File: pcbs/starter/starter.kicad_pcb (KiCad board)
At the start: 2 copper layers, 62.5 x 68.5 mm, 17 parts, among them J1 Conn_01x06_Socket, J2 Relay Anschluss, J3 12V Eingang und GND, J4 Conn_01x02_Socket, Q2 2N7000, Q3 2N7000, Q4 2N7000, U1 ESP32-C3_SUPERMINI_TH

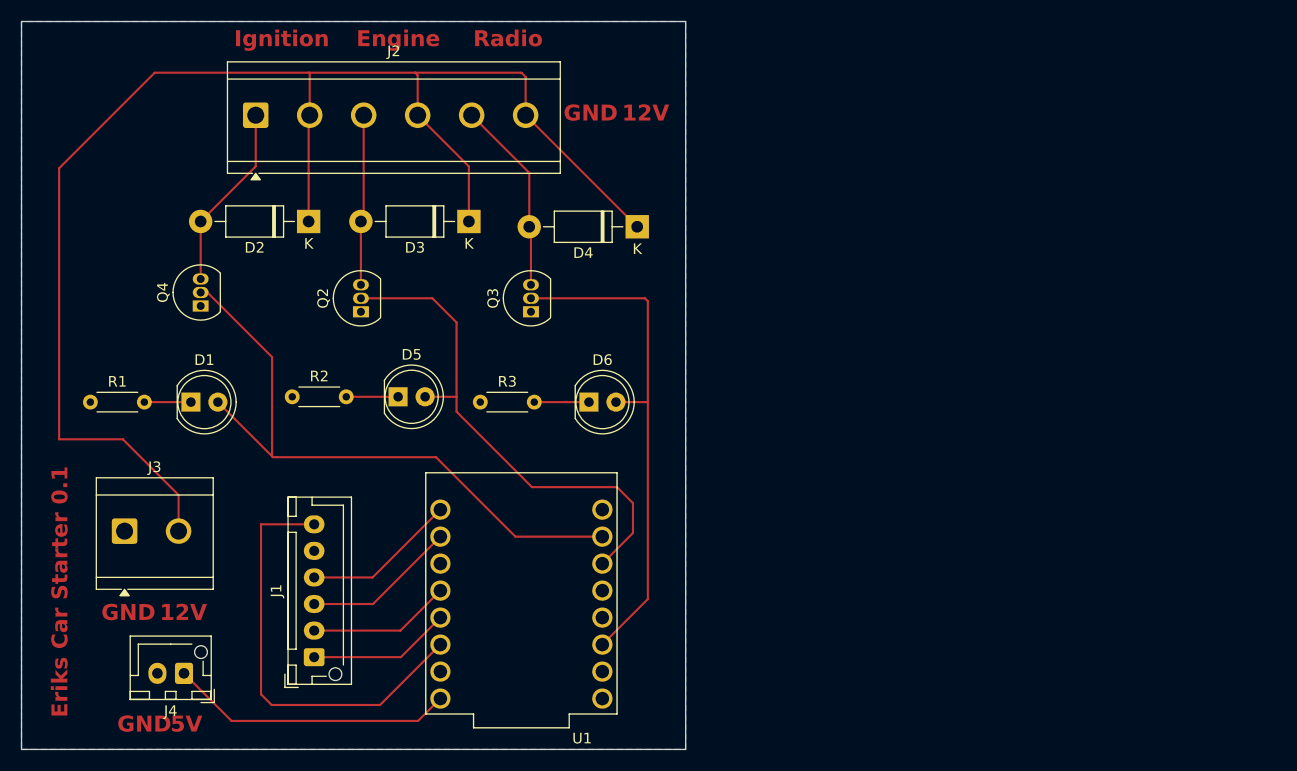
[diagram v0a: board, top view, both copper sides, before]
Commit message: first pcb revision ordered at JLCPCB
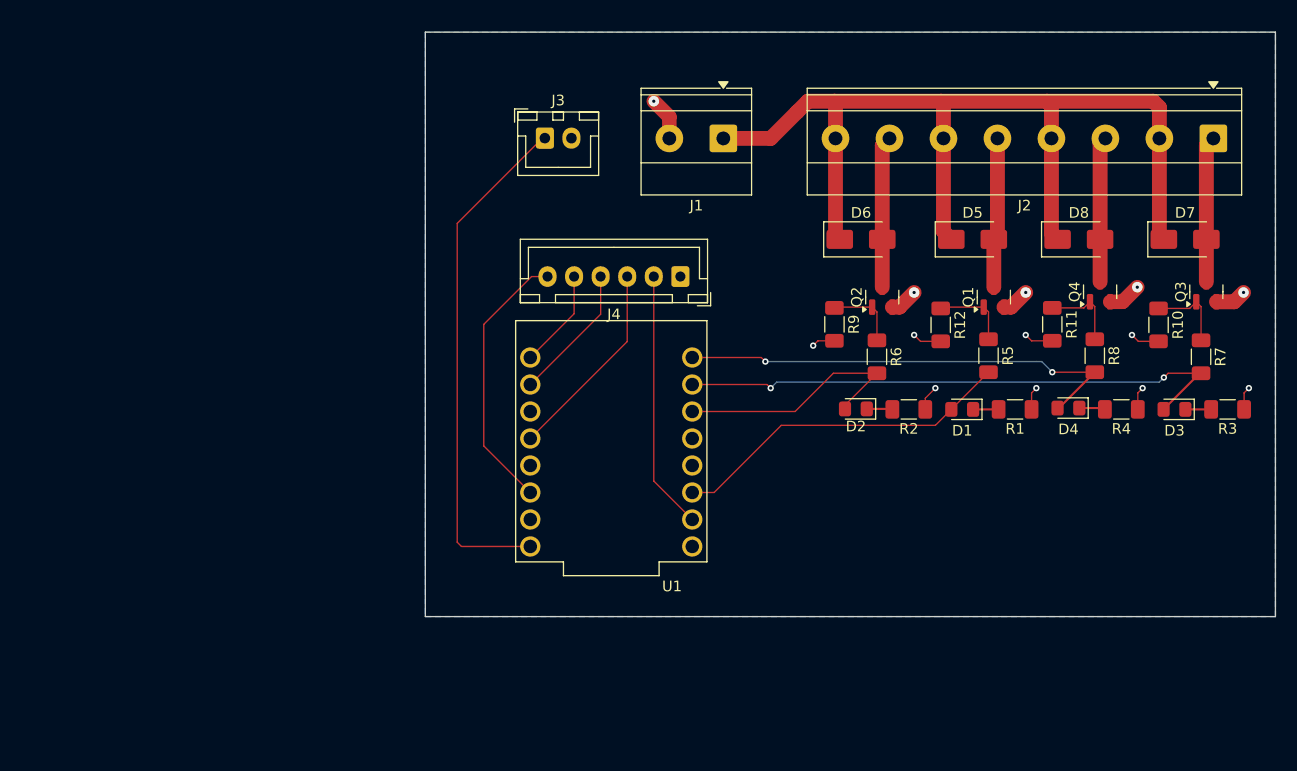
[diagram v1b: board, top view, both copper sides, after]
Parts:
- added D7: SS14, Diode_SMD:D_SMA, F.Cu at (189.0, 69.0)
- added D8: SS14, Diode_SMD:D_SMA, F.Cu at (179.0, 69.0)
- added Q1: AO3400A, Package_TO_SOT_SMD:SOT-23, F.Cu at (171.0, 74.4)
- added R10: 10k, Resistor_SMD:R_1206_3216Metric_Pad1.30x1.75mm_HandSolder, F.Cu at (186.5, 77.0)
- added R11: 10k, Resistor_SMD:R_1206_3216Metric_Pad1.30x1.75mm_HandSolder, F.Cu at (176.5, 77.0)
- added R12: 10k, Resistor_SMD:R_1206_3216Metric_Pad1.30x1.75mm_HandSolder, F.Cu at (166.0, 77.0)
- added R4: 200, Resistor_SMD:R_1206_3216Metric_Pad1.30x1.75mm_HandSolder, F.Cu at (183.0, 85.0)
- added R5: 47, Resistor_SMD:R_1206_3216Metric_Pad1.30x1.75mm_HandSolder, F.Cu at (170.5, 80.0)
- added R6: 47, Resistor_SMD:R_1206_3216Metric_Pad1.30x1.75mm_HandSolder, F.Cu at (160.0, 80.0)
- added R7: 47, Resistor_SMD:R_1206_3216Metric_Pad1.30x1.75mm_HandSolder, F.Cu at (190.5, 80.0)
- added R8: 47, Resistor_SMD:R_1206_3216Metric_Pad1.30x1.75mm_HandSolder, F.Cu at (180.5, 80.0)
- added R9: 10k, Resistor_SMD:R_1206_3216Metric_Pad1.30x1.75mm_HandSolder, F.Cu at (156.0, 77.0)
- D1: footprint LED_THT:LED_D5.0mm -> LED_SMD:LED_0805_2012Metric_Pad1.15x1.40mm_HandSolder
- D2, D3, D4: value 1N4003 -> LED; footprint Diode_THT:D_DO-41_SOD81_P10.16mm_Horizontal -> LED_SMD:LED_0805_2012Metric_Pad1.15x1.40mm_HandSolder
- D5, D6: value LED -> SS14; footprint LED_THT:LED_D5.0mm -> Diode_SMD:D_SMA
- J1: value Conn_01x06_Socket -> Power 12V; footprint Connector_JST:JST_XH_B6B-XH-AM_1x06_P2.50mm_Vertical -> TerminalBlock_Phoenix:TerminalBlock_Phoenix_MKDS-1,5-2-5.08_1x02_P5.08mm_Horizontal
- J2: value Relay Anschluss -> Relays; footprint TerminalBlock_CUI:TerminalBlock_CUI_TB007-508-06_1x06_P5.08mm_Horizontal -> TerminalBlock_Phoenix:TerminalBlock_Phoenix_MKDS-1,5-8-5.08_1x08_P5.08mm_Horizontal
- J3: value 12V Eingang und GND -> Power 5V; footprint TerminalBlock_CUI:TerminalBlock_CUI_TB007-508-02_1x02_P5.08mm_Horizontal -> Connector_JST:JST_XH_B2B-XH-A_1x02_P2.50mm_Vertical
- J4: value Conn_01x02_Socket -> Sensor Key Position; footprint Connector_JST:JST_XH_B2B-XH-AM_1x02_P2.50mm_Vertical -> Connector_JST:JST_XH_B6B-XH-A_1x06_P2.50mm_Vertical
- Q2, Q3, Q4: value 2N7000 -> AO3400A; footprint Package_TO_SOT_THT:TO-92_Inline -> Package_TO_SOT_SMD:SOT-23
- R1, R2, R3: value 200R -> 200; footprint Resistor_THT:R_Axial_DIN0204_L3.6mm_D1.6mm_P5.08mm_Horizontal -> Resistor_SMD:R_1206_3216Metric_Pad1.30x1.75mm_HandSolder
- moved J2 90.1 mm to (191.7, 59.5), turned to 180 degrees
- moved R1 87.0 mm to (173.0, 85.0), turned to 180 degrees
- moved Q4 84.7 mm to (181.0, 73.9)
- moved D1 72.6 mm to (168.0, 85.0), turned to 180 degrees
- moved R3 70.3 mm to (193.0, 85.0), turned to 180 degrees
- moved D3 68.7 mm to (188.0, 85.0)
- moved Q3 63.6 mm to (191.0, 73.9)
- moved J1 62.2 mm to (145.5, 59.5), turned to 180 degrees
- moved J4 59.8 mm to (141.5, 72.5)
- moved R2 58.0 mm to (163.0, 85.0), turned to 180 degrees
- moved D5 56.1 mm to (169.0, 69.0)
- moved D2 54.4 mm to (158.0, 85.0)
- moved J3 54.1 mm to (128.8, 59.5)
- moved Q2 49.1 mm to (160.5, 74.4)
- moved D4 44.0 mm to (178.0, 84.9)
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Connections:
- D2 pad 1: +12V -> Net-(D2-K)
- D3 pad 1: +12V -> Net-(D3-K)
- D4 pad 1: +12V -> Net-(D4-K)
- D5 pad 1: Net-(D5-K) -> +12V
- D6 pad 1: Net-(D6-K) -> +12V
- J1 pad 1: Net-(J1-Pin_1) -> +12V
- J1 pad 2: Net-(J1-Pin_2) -> GND
- J2 pad 1: Net-(D2-A) -> Net-(D7-A)
- J2 pad 3: Net-(D3-A) -> Net-(D8-A)
- J2 pad 5: Net-(D4-A) -> Net-(D5-A)
- J3 pad 1: GND -> +5V
- J3 pad 2: +12V -> GND
- J4 pad 1: +5V -> unconnected-(J4-Pin_1-Pad1)
- J4 pad 2: GND -> Net-(J4-Pin_2)
- Q2 pad 1: GND -> Net-(Q2-G)
- Q2 pad 2: Net-(D5-A) -> GND
- Q2 pad 3: Net-(D3-A) -> Net-(D6-A)
- Q3 pad 1: GND -> Net-(Q3-G)
- Q3 pad 2: Net-(D6-A) -> GND
- Q3 pad 3: Net-(D4-A) -> Net-(D7-A)
- Q4 pad 1: GND -> Net-(Q4-G)
- Q4 pad 2: Net-(D1-A) -> GND
- Q4 pad 3: Net-(D2-A) -> Net-(D8-A)
- R2 pad 2: Net-(D5-K) -> Net-(D2-K)
- R3 pad 2: Net-(D6-K) -> Net-(D3-K)
- U1 pad 0: Net-(J1-Pin_4) -> Net-(J4-Pin_5)
- U1 pad 1: Net-(J1-Pin_3) -> Net-(J4-Pin_4)
- U1 pad 10: Net-(D5-A) -> Net-(D2-A)
- U1 pad 20: Net-(D1-A) -> Net-(D3-A)
- U1 pad 21: unconnected-(U1-GPIO21-Pad21) -> Net-(D4-A)
- U1 pad 3: Net-(J1-Pin_2) -> Net-(J4-Pin_3)
- U1 pad 3.3: +3.3V -> Net-(J4-Pin_6)
- U1 pad 4: Net-(J1-Pin_1) -> unconnected-(U1-GPIO4-Pad4)
- U1 pad 6: unconnected-(U1-GPIO6-Pad6) -> Net-(J4-Pin_2)
- U1 pad 7: Net-(D6-A) -> Net-(D1-A)
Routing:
- net +12V: track 138.9 -> 95.4 mm
- net +3.3V: track 40.6 -> 0.00 mm
- net Net-(D3-A): track 16.1 -> 53.5 mm, vias 0 -> 2
- net Net-(D6-A): track 49.4 -> 14.3 mm
- net GND: track 0.00 -> 34.7 mm, vias 0 -> 13
- net Net-(D5-A): track 48.4 -> 14.1 mm
- net Net-(D1-A): track 60.0 -> 33.1 mm
- net Net-(J4-Pin_6): track 0.00 -> 25.5 mm
- net Net-(D4-A): track 18.3 -> 43.4 mm, vias 0 -> 2
- net Net-(J4-Pin_2): track 0.00 -> 24.4 mm
- net +5V: track 26.9 -> 48.6 mm
- net Net-(J4-Pin_3): track 0.00 -> 19.0 mm
- net Net-(J1-Pin_4): track 14.5 -> 0.00 mm
- net Net-(J1-Pin_3): track 14.5 -> 0.00 mm
- net Net-(J1-Pin_1): track 14.2 -> 0.00 mm
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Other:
- board size 62.5 x 68.5 mm -> 80 x 55 mm
- copper layers 2 -> 4
- board text removed: "12V"
- board text removed: "5V"
- board text removed: "Engine"
- board text removed: "Eriks Car Starter 0.1"
- board text removed: "GND"
- board text removed: "Ignition"
- board text removed: "Radio"
